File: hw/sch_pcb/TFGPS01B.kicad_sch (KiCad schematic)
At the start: 72 parts, among them J1 SM10B-GHS-TB, J2 USBC_USB4105-GF-A, J3 SM06B-GHS-TB, J4 SM04B-GHS-TB, J5 SM08B-GHS-TB, M1 HOLE, M2 HOLE, M3 HOLE, M4 HOLE, Q1 BC817-25, Q2 BC817-25, Q3 BC817-25, U1 MIC5504-3.3YM5, U2 USBLC6-2SC6, U3 NEO-M8P, U4 MAX2655

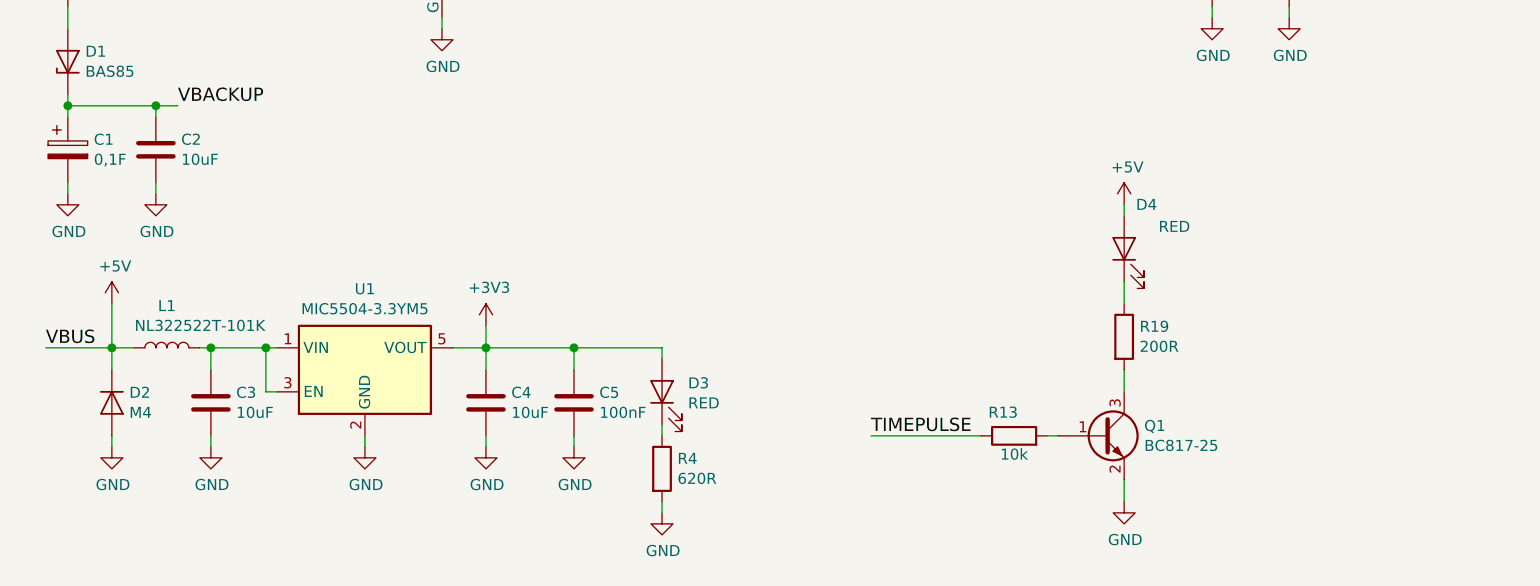
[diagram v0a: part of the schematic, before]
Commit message: Edit schema
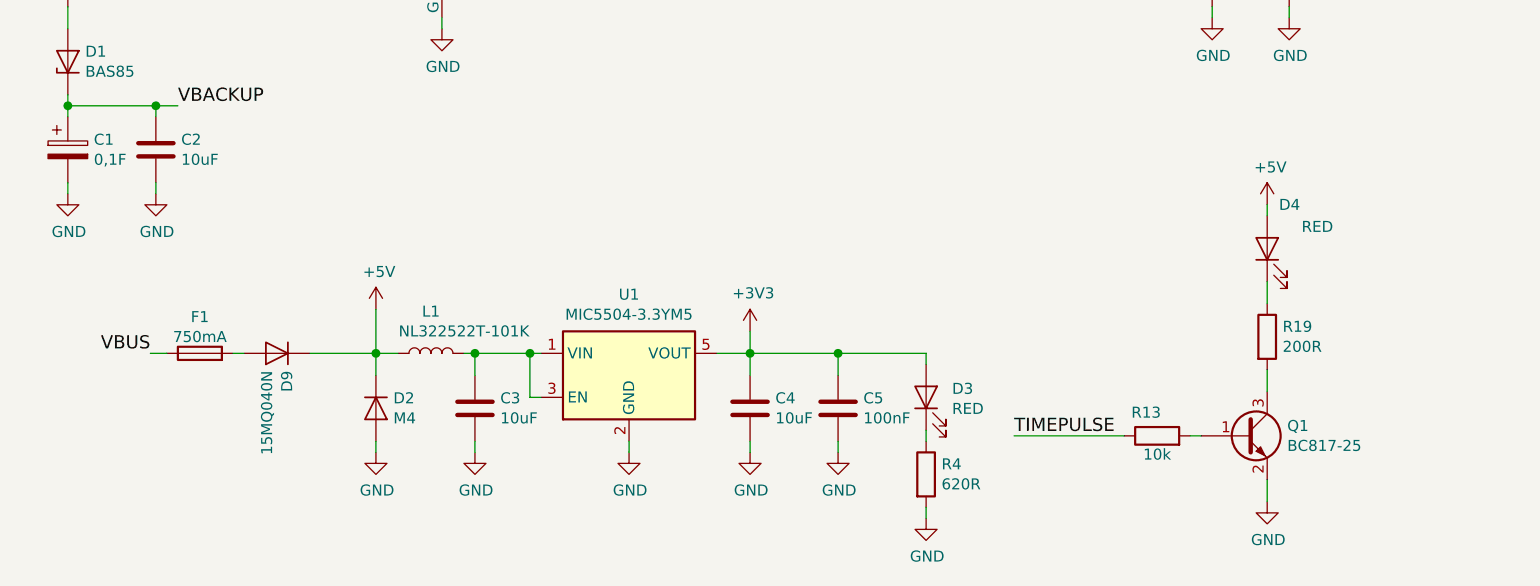
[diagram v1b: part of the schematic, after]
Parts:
- added D9: 15MQ040N, Diode_SMD:D_SMA, symbol Device:D
- added F1: 750mA, Fuse:Fuse_0805_2012Metric, symbol Device:Fuse
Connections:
- net +5V: now also D9.1 (K); no longer J2.A4/B9 (VBUS), J2.B4/A9 (VBUS), U2.5 (VBUS)
- new net: D9.2 (A), F1.2
- new net VBUS: F1.1, J2.A4/B9 (VBUS), J2.B4/A9 (VBUS), U2.5 (VBUS)
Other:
- moved on the sheet: C3, C4, C5, D2, D3, D4, L1, Q1, R13, R19, R4, U1
